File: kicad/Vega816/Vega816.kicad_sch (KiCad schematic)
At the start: 0 parts

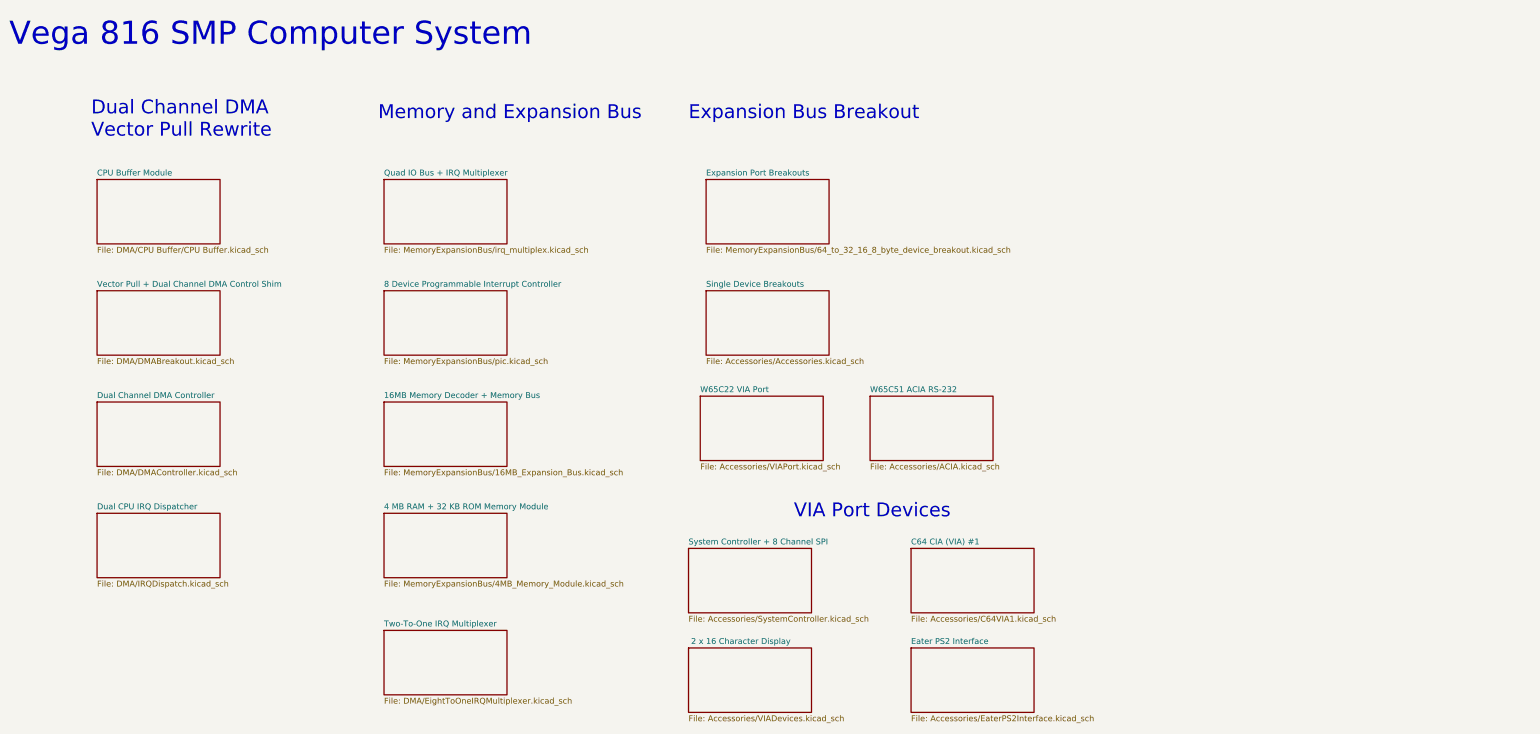
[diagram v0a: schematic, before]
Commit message: var
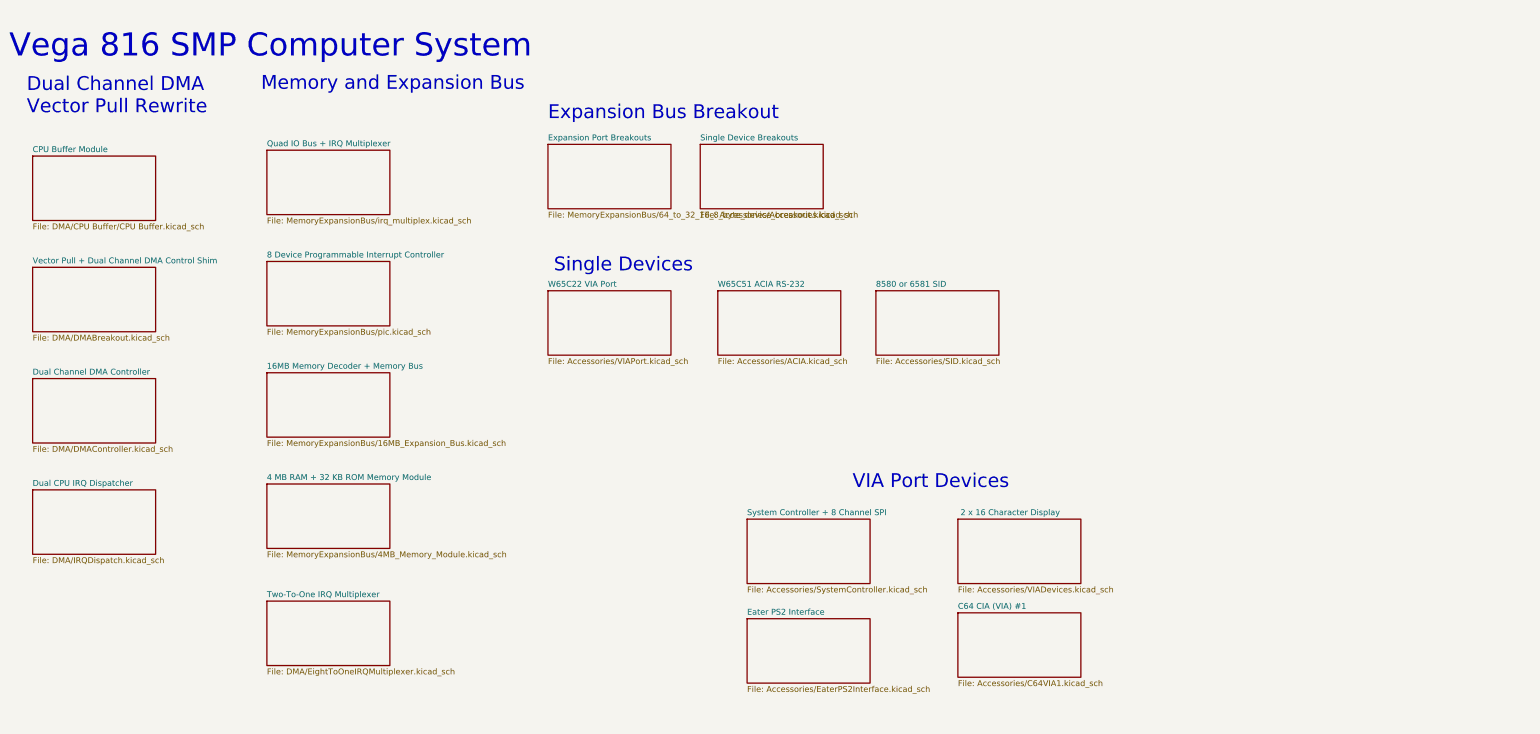
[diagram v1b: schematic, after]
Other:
- added sheet 8580 or 6581 SID (Accessories/SID.kicad_sch)
- note added: "Single Devices"

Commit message: update
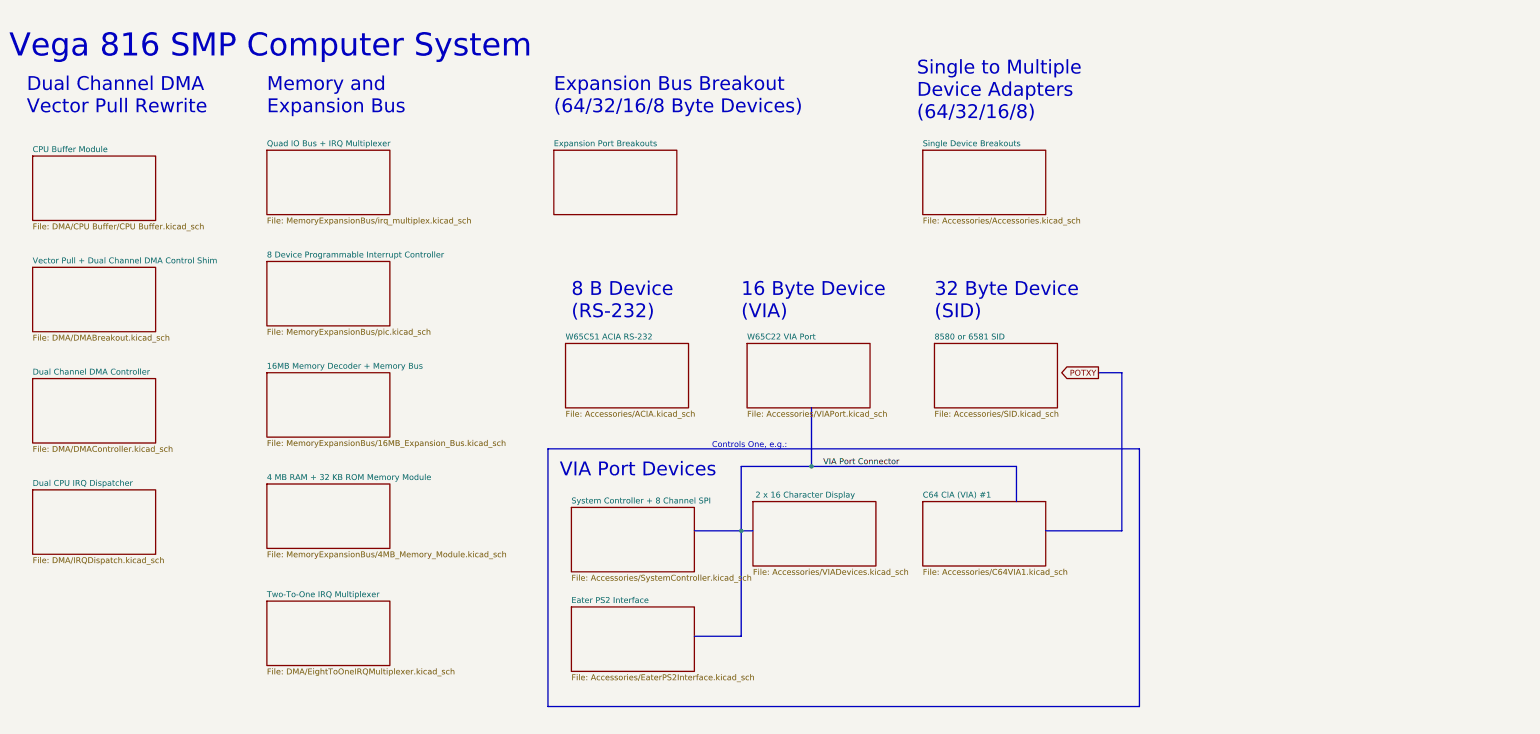
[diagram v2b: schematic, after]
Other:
- note added: "16 Byte Device (VIA)"
- note added: "32 Byte Device (SID)"
- note added: "8 B Device (RS-232)"
- note added: "Controls One, e.g.:"
- note added: "Expansion Bus Breakout (64/32/16/8 Byte Devices)"
- note added: "Single to Multiple Device Adapters (64/32/16/8)"
- note removed: "Expansion Bus Breakout"
- note removed: "Single Devices"

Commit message: irq
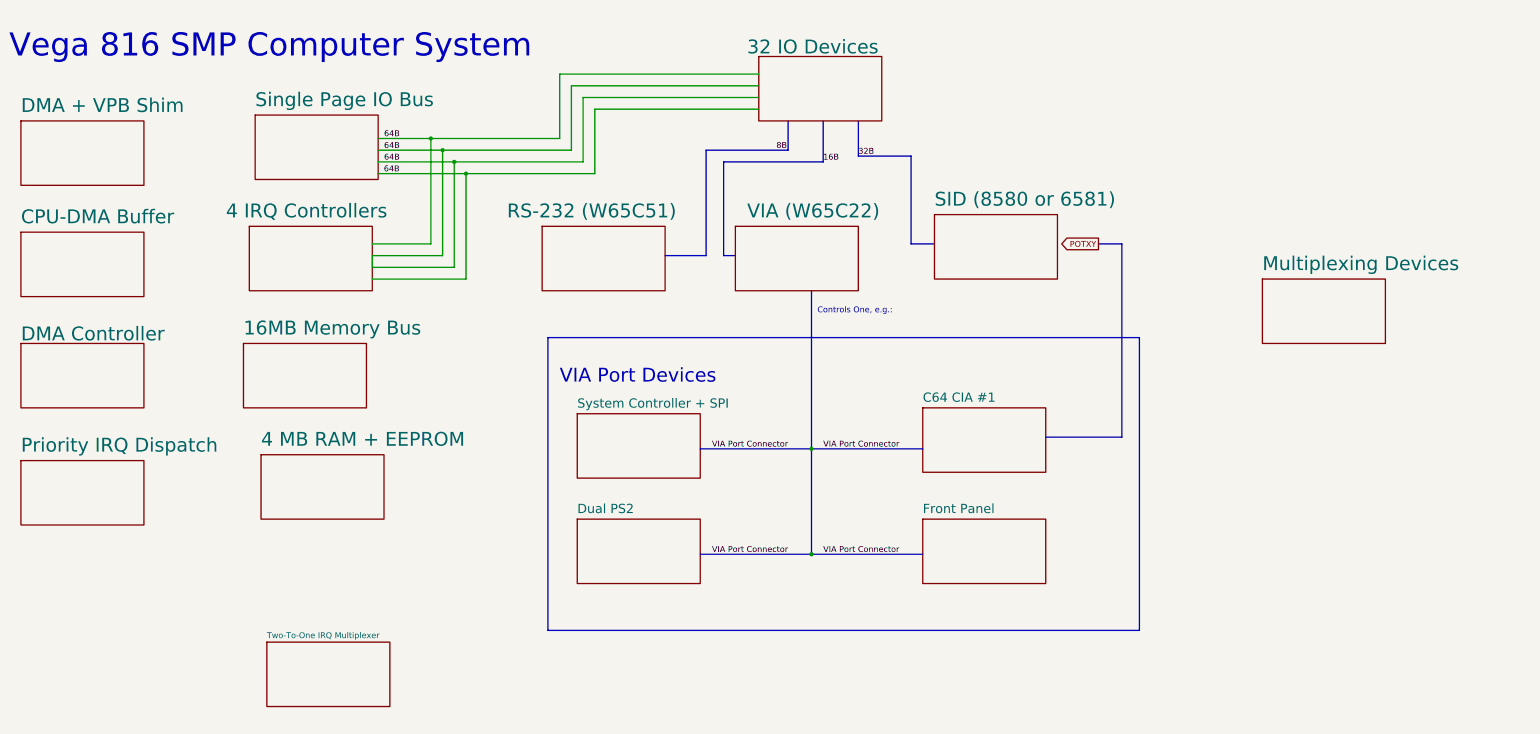
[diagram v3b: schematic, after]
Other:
- sheet  2 x 16 Character Display renamed Front Panel
- sheet 16MB Memory Decoder + Memory Bus renamed 16MB Memory Bus
- sheet 4 MB RAM + 32 KB ROM Memory Module renamed 4 MB RAM + EEPROM
- sheet 8 Device Programmable Interrupt Controller renamed 4 IRQ Controllers
- sheet 8580 or 6581 SID renamed SID (8580 or 6581)
- sheet C64 CIA (VIA) #1 renamed C64 CIA #1
- sheet CPU Buffer Module renamed CPU-DMA Buffer
- sheet Dual CPU IRQ Dispatcher renamed Priority IRQ Dispatch
- sheet Dual Channel DMA Controller renamed DMA Controller
- sheet Eater PS2 Interface renamed Dual PS2
- sheet Expansion Port Breakouts renamed 32 IO Devices
- sheet Quad IO Bus + IRQ Multiplexer renamed Single Page IO Bus
- sheet Single Device Breakouts renamed Multiplexing Devices
- sheet System Controller + 8 Channel SPI renamed System Controller + SPI
- sheet Vector Pull + Dual Channel DMA Control Shim renamed DMA + VPB Shim
- sheet W65C22 VIA Port renamed VIA (W65C22)
- sheet W65C51 ACIA RS-232 renamed RS-232 (W65C51)
- note removed: "16 Byte Device (VIA)"
- note removed: "32 Byte Device (SID)"
- note removed: "8 B Device (RS-232)"
- note removed: "Dual Channel DMA Vector Pull Rewrite"
- note removed: "Expansion Bus Breakout (64/32/16/8 Byte Devices)"
- note removed: "Memory and Expansion Bus"
- note removed: "Single to Multiple Device Adapters (64/32/16/8)"
